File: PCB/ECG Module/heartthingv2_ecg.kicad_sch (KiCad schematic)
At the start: 30 parts, among them J1 Conn_01x09_Socket, J2 Conn_01x03_Socket, U1 TXB0108PW, U2 MAX30003CTI_, U3 AP2112K-1.8

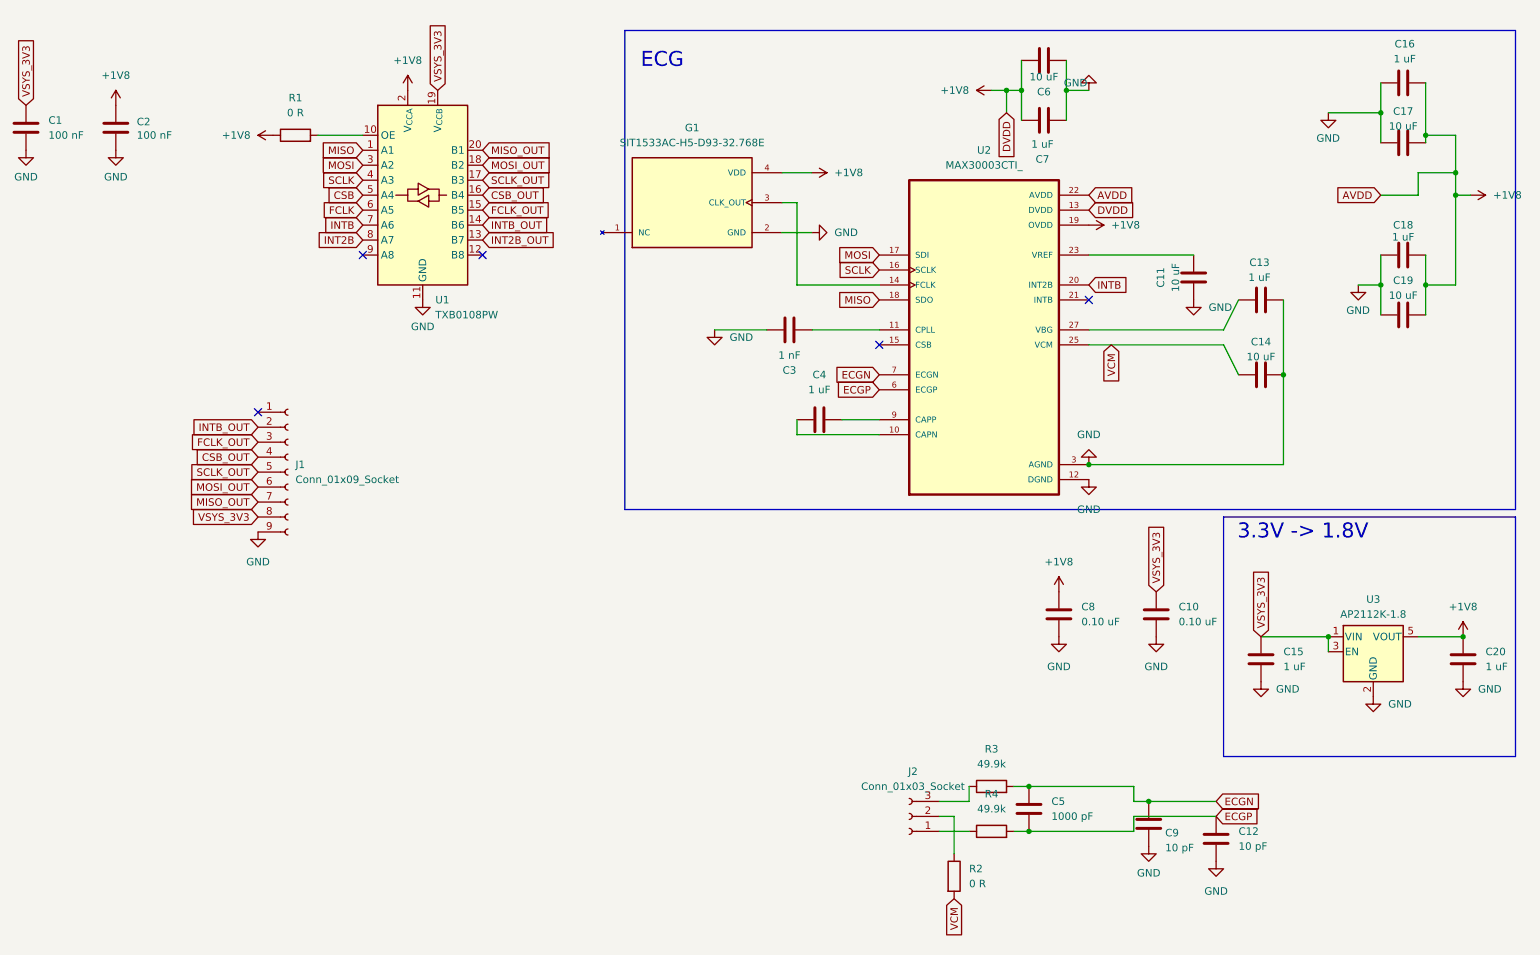
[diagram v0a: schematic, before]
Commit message: jogeshwari
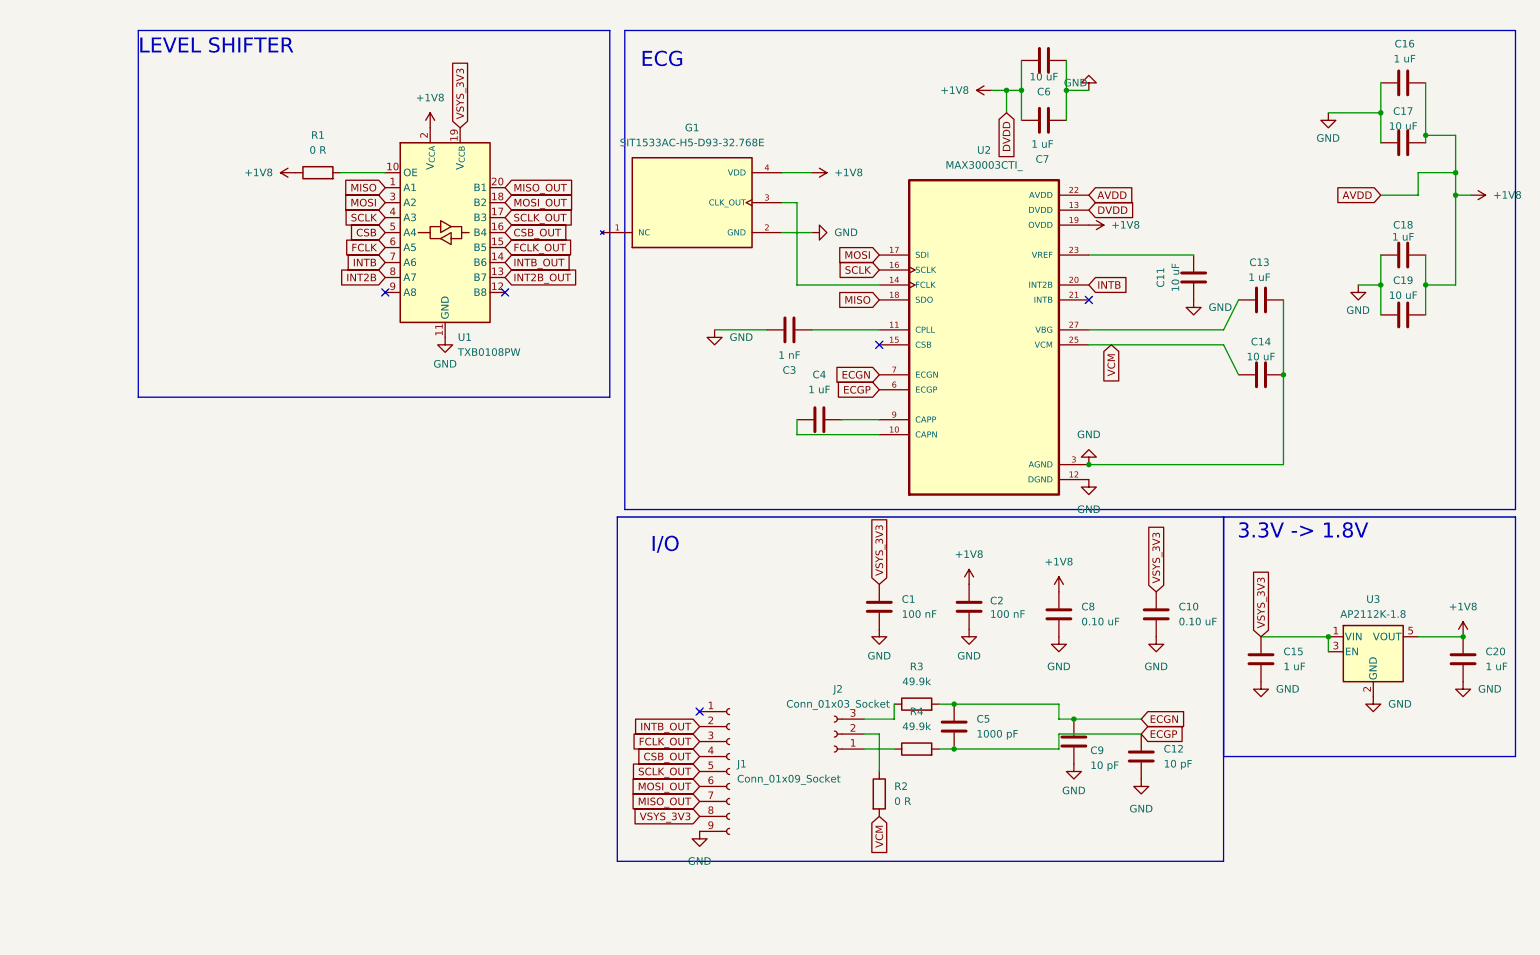
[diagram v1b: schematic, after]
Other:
- note added: "I/O"
- note added: "LEVEL SHIFTER"
- moved on the sheet: C1, C12, C2, C5, C9, J1, J2, R1, R2, R3, R4, U1
